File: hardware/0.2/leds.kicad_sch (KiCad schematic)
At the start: 16 parts, among them Q501 BSS138, Q502 BSS138, Q503 BSS138

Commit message: checking for the final time
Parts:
- R510, R513, R515: MPN RC0402JR-0710KL -> RC0402JR-0710KL
- RN500, RN501: MPN YC164-JR-07220RL -> YC124-JR-07220RL
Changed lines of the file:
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@@
       (effects (font (size 1.27 1.27)) hide)
     )
-    (property "MPN" "YC164-JR-07220RL" (id 5) (at 92.71 82.55 0)
+    (property "MPN" "YC124-JR-07220RL\n" (id 5) (at 92.71 82.55 0)
       (effects (font (size 1.27 1.27)) hide)
     )
@@
       (effects (font (size 1.27 1.27)) hide)
     )
-    (property "MPN" "YC164-JR-07220RL" (id 5) (at 111.76 82.55 0)
+    (property "MPN" "YC124-JR-07220RL\n" (id 5) (at 111.76 82.55 0)
       (effects (font (size 1.27 1.27)) hide)
     )
@@
       (effects (font (size 1.27 1.27)) hide)
     )
-    (property "MPN" "YC164-JR-07220RL" (id 5) (at 130.81 82.55 0)
+    (property "MPN" "YC124-JR-07220RL\n" (id 5) (at 130.81 82.55 0)
       (effects (font (size 1.27 1.27)) hide)
     )
@@
       (effects (font (size 1.27 1.27)) hide)
     )
-    (property "MPN" "YC164-JR-07220RL" (id 5) (at 149.86 82.55 0)
+    (property "MPN" "YC124-JR-07220RL\n" (id 5) (at 149.86 82.55 0)
       (effects (font (size 1.27 1.27)) hide)
     )
@@
       (effects (font (size 1.27 1.27)) hide)
     )
-    (property "MPN" "YC164-JR-07220RL" (id 5) (at 168.91 82.55 0)
+    (property "MPN" "YC124-JR-07220RL\n" (id 5) (at 168.91 82.55 0)
       (effects (font (size 1.27 1.27)) hide)
     )
@@
       (effects (font (size 1.27 1.27)) hide)
     )
-    (property "MPN" "YC164-JR-07220RL" (id 5) (at 187.96 82.55 0)
+    (property "MPN" "YC124-JR-07220RL\n" (id 5) (at 187.96 82.55 0)
       (effects (font (size 1.27 1.27)) hide)
     )
@@
       (effects (font (size 1.27 1.27)) hide)
     )
-    (property "MPN" "YC164-JR-07220RL" (id 5) (at 207.01 82.55 0)
+    (property "MPN" "YC124-JR-07220RL\n" (id 5) (at 207.01 82.55 0)
       (effects (font (size 1.27 1.27)) hide)
     )
@@
       (effects (font (size 1.27 1.27)) hide)
     )
-    (property "MPN" "YC164-JR-07220RL" (id 5) (at 226.06 82.55 0)
+    (property "MPN" "YC124-JR-07220RL\n" (id 5) (at 226.06 82.55 0)
       (effects (font (size 1.27 1.27)) hide)
     )
@@
       (effects (font (size 1.27 1.27)) hide)
     )
-    (property "MPN" "RC0402JR-0710KL" (id 5) (at 123.19 130.81 0)
+    (property "MPN" "RC0402JR-0710KL\n" (id 5) (at 123.19 130.81 0)
       (effects (font (size 1.27 1.27)) hide)
     )
@@
       (effects (font (size 1.27 1.27)) hide)
     )
-    (property "MPN" "RC0402JR-0710KL" (id 5) (at 153.67 130.81 0)
+    (property "MPN" "RC0402JR-0710KL\n" (id 5) (at 153.67 130.81 0)
       (effects (font (size 1.27 1.27)) hide)
     )
@@
       (effects (font (size 1.27 1.27)) hide)
     )
-    (property "MPN" "RC0402JR-0710KL" (id 5) (at 181.61 130.81 0)
-      (effects (font (size 1.27 1.27)) hide)
-    )
+    (property "MPN" "RC0402JR-0710KL\n" (id 5) (at 181.61 130.81 0)
+      (effects (font (size 1.27 1.27)) hide)
+    )

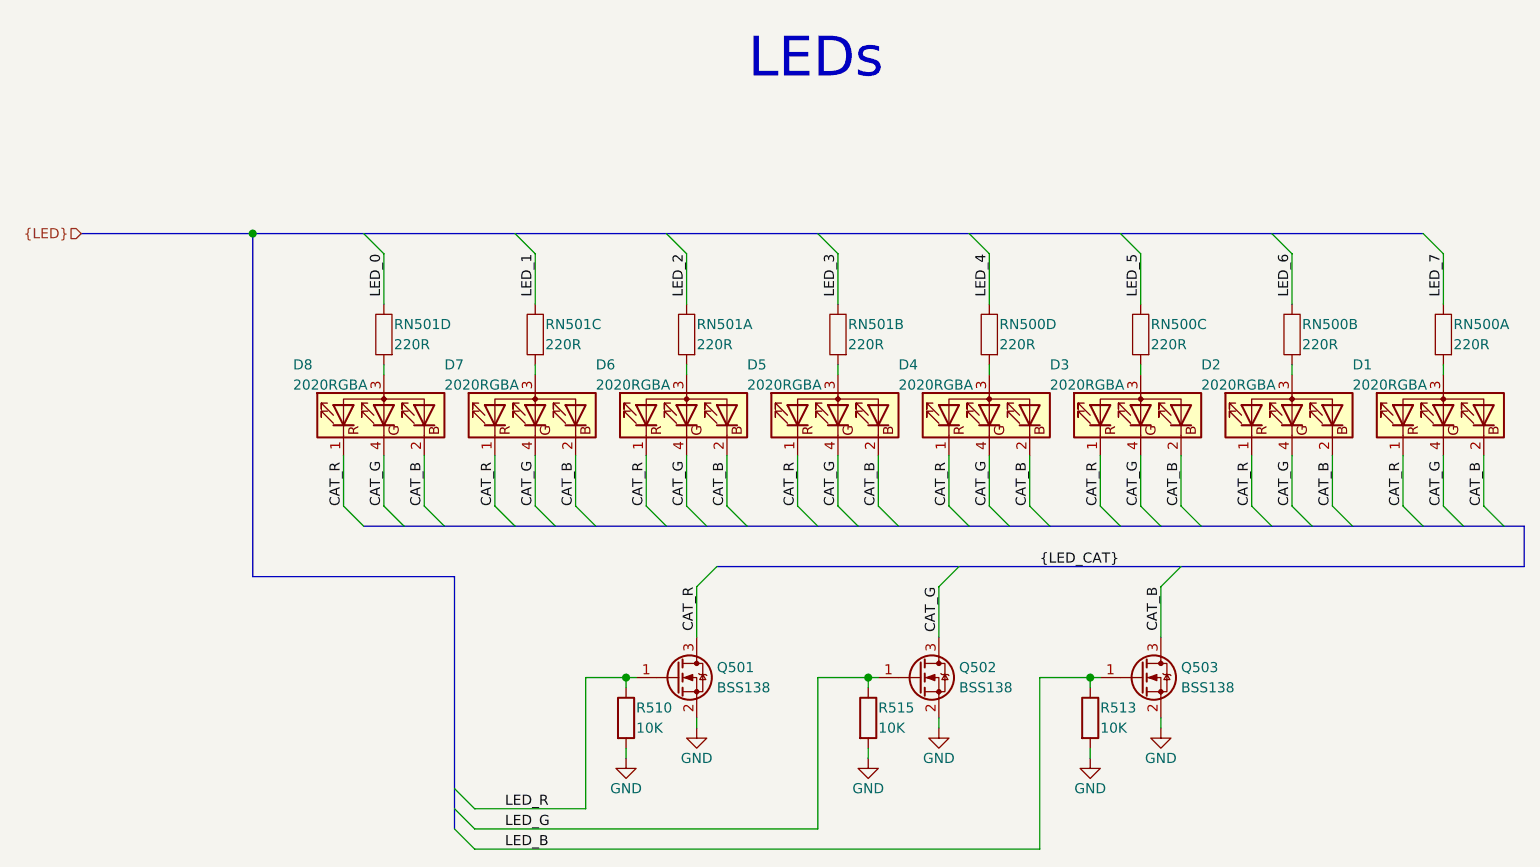
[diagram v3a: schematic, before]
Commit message: nightly version bump
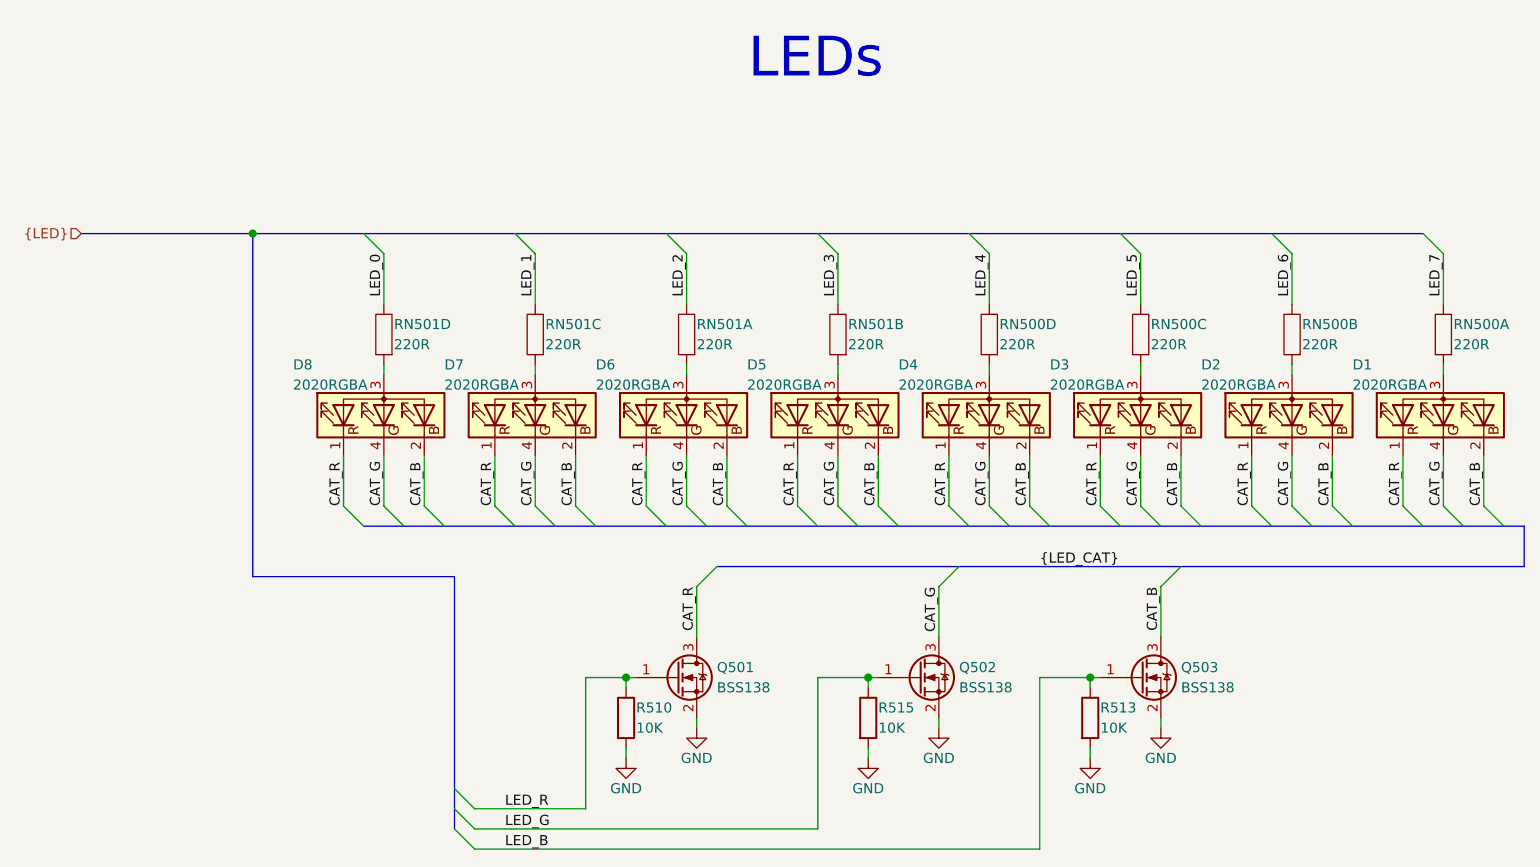
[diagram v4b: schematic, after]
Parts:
- Q501, Q502, Q503: MPN2 BSS138W-7-F -> (none)
- R510, R513, R515: MPN2 0402WGJ0103TCE -> (none)
- RN500, RN501: MPN2 4D02WGJ0221TCE -> (none)
